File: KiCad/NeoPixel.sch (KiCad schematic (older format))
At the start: 0 parts

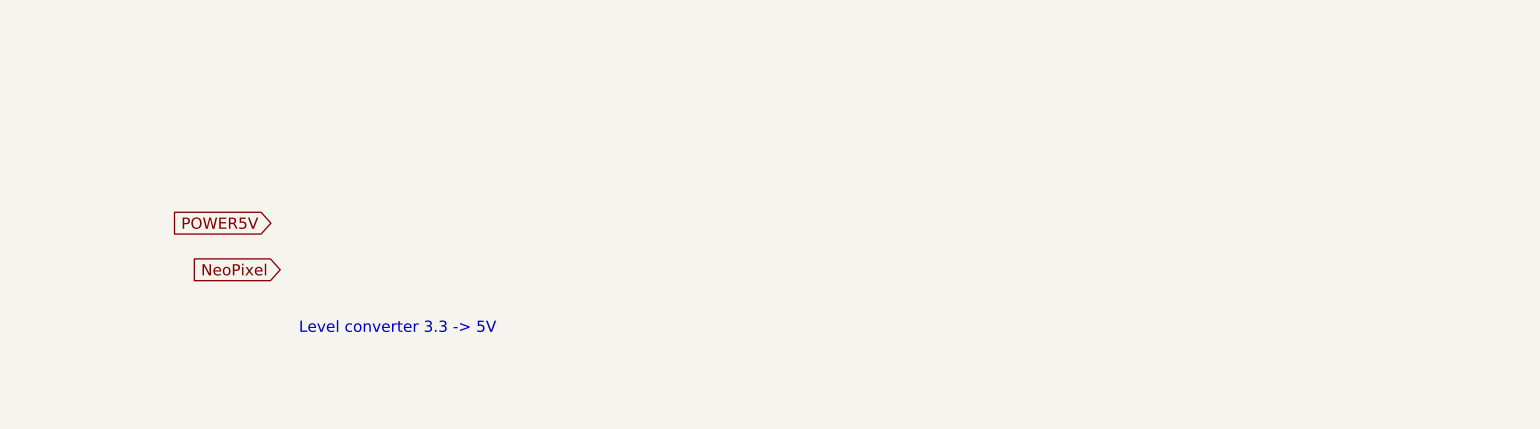
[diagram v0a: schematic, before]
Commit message: More work
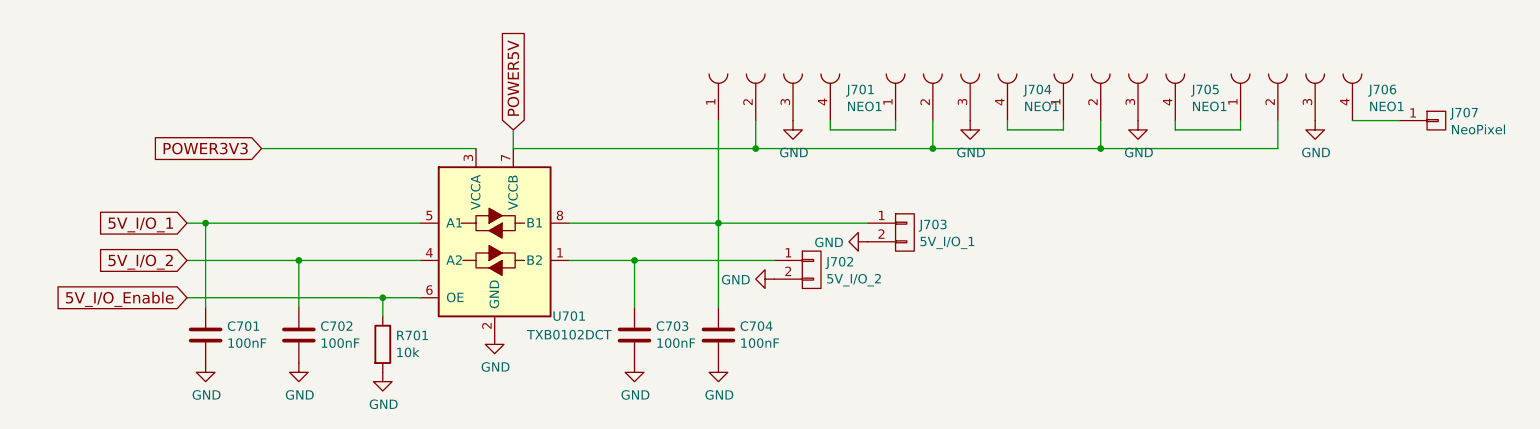
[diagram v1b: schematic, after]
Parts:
- added C701, C702, C703, C704: 100nF, Capacitors_SMD:C_0805, symbol C
- added J701, J704, J705, J706: NEO1, Pin_Headers:Pin_Header_Straight_1x04_Pitch1.27mm, symbol CONN_01X04_FEMALE
- added J702: 5V_I/O_2, Pin_Headers:Pin_Header_Straight_1x02_Pitch2.54mm, symbol CONN_01X02
- added J703: 5V_I/O_1, Pin_Headers:Pin_Header_Straight_1x02_Pitch2.54mm, symbol CONN_01X02
- added J707: NeoPixel, Pin_Headers:Pin_Header_Straight_1x01_Pitch2.54mm, symbol CONN_01X01
- added R701: 10k, Resistors_SMD:R_0805, symbol R
- added U701: TXB0102DCT, Housings_SSOP:TSSOP-8_3x3mm_Pitch0.65mm, symbol TXB0102DCT
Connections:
- net POWER5V: now also J701.2, J704.2, J705.2, J706.2, U701.7 (VCCB)
- new net: C703.1, J702.1 (P1), U701.1 (B2)
- new net: C704.1, J701.1, J703.1 (P1), U701.8 (B1)
- new net: J701.4, J704.1
- new net: J704.4, J705.1
- new net: J705.4, J706.1
- new net: J706.4, J707.1 (P1)
- new net 5V_I/O_1: C701.1, U701.5 (A1)
- new net 5V_I/O_2: C702.1, U701.4 (A2)
- new net 5V_I/O_Enable: R701.1, U701.6 (OE)
- new net GND: C701.2, C702.2, C703.2, C704.2, J701.3, J702.2 (P2), J703.2 (P2), J704.3, J705.3, J706.3, R701.2, U701.2 (GND)
- new net POWER3V3: U701.3 (VCCA)
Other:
- note removed: "Level converter 3.3 -> 5V"
